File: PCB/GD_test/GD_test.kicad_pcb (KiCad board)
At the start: 2 copper layers, 46 x 51.3 mm, 47 parts, among them J1 RF_IN, J2 RF_IN, J3 RF_IN, J4 RF_IN, J5 Conn_01x01_Pin, J6 Conn_01x01_Pin, Q1 EPC2051, Q2 EPC2051, Q3 EPC2070, Q5 EPC2014C, U1 LMG1020YFF, U10 TLV3501, U11 LMG1020YFF, U2 TLV3501, U3 NC7WZ04, U4 TLV3501, U5 NC7WZ04, U6 NC7WZ04, U7 NC7WZ04, U8 TLV3501, U9 LMG1020YFF

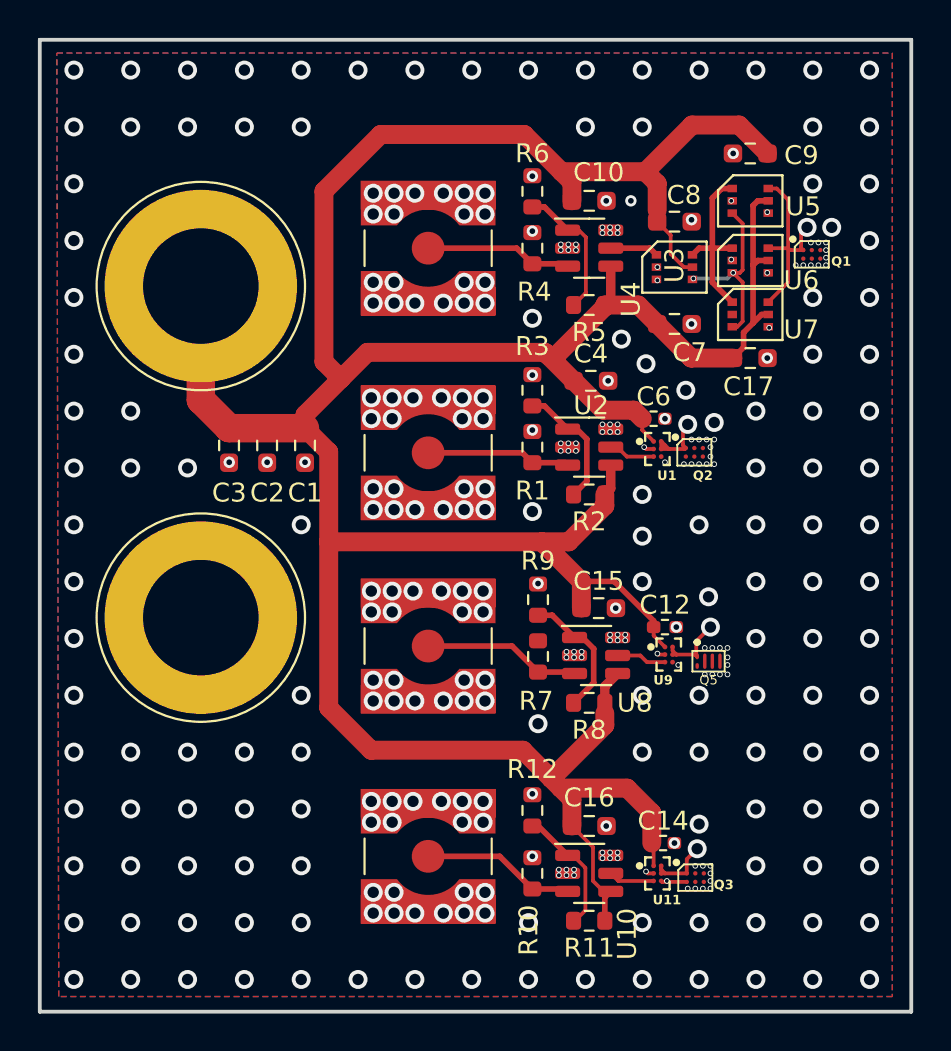
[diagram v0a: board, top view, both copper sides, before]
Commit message: gate driver gerbers and some extra changes
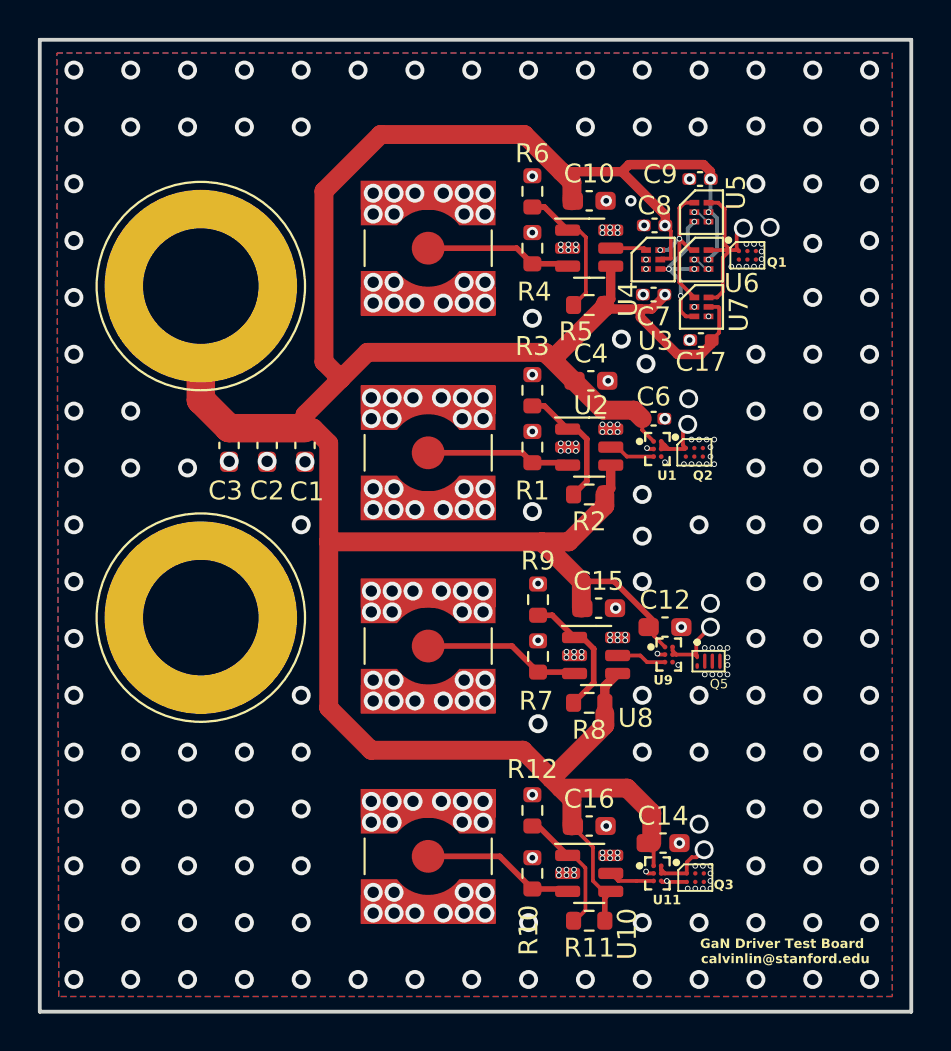
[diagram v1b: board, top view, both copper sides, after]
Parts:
- C1, C10, C15, C16, C2, C3, C4: footprint Resistor_SMD:R_0603_1608Metric_Pad0.98x0.95mm_HandSolder -> Capacitor_SMD:C_0603_1608Metric_Pad1.08x0.95mm_HandSolder
- C12, C14: footprint Resistor_SMD:R_0402_1005Metric_Pad0.72x0.64mm_HandSolder -> Capacitor_SMD:C_0603_1608Metric_Pad1.08x0.95mm_HandSolder
- C17, C7, C8, C9: footprint Resistor_SMD:R_0603_1608Metric_Pad0.98x0.95mm_HandSolder -> Capacitor_SMD:C_0402_1005Metric_Pad0.74x0.62mm_HandSolder
- C6: footprint Resistor_SMD:R_0402_1005Metric_Pad0.72x0.64mm_HandSolder -> Capacitor_SMD:C_0402_1005Metric_Pad0.74x0.62mm_HandSolder
- moved Q1 3.40 mm to (140.3, 76.9)
- moved C9 2.97 mm to (137.8, 72.8)
- moved C17 2.77 mm to (137.9, 81.3), turned to 180 degrees
- moved U5 2.64 mm to (137.9, 74.6)
- moved U7 2.61 mm to (137.9, 79.6)
- moved U6 2.58 mm to (137.9, 77.1)
- moved C7 1.90 mm to (135.4, 79.0), turned to 180 degrees
- moved U3 1.19 mm to (135.4, 77.1)
- moved C8 1.07 mm to (135.4, 75.3), turned to 180 degrees
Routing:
- net +5V: track 192.4 -> 186.2 mm, vias 0 -> 5
- net GND: track 2.77 -> 4.52 mm, vias 335 -> 341
- net /BUFF_OUT+: track 9.44 -> 8.25 mm, vias 0 -> 2
- net /BUFF_OUT-: track 9.45 -> 8.34 mm, vias 2 -> 4
- net Net-(Q1-G): track 10.4 -> 9.54 mm
- net Net-(U3-A1): track 2.56 -> 1.90 mm
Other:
- board text added: "GaN Driver Test Board"
- board text added: "calvinlin@stanford.edu"
